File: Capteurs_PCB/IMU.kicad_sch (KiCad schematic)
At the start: 3 parts, among them U3 LSM6DSL

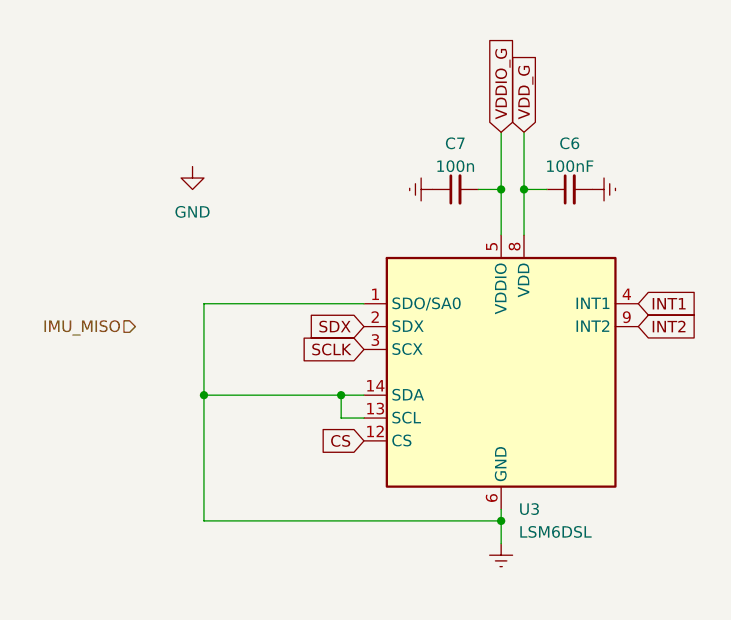
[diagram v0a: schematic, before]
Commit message: Modif PCB
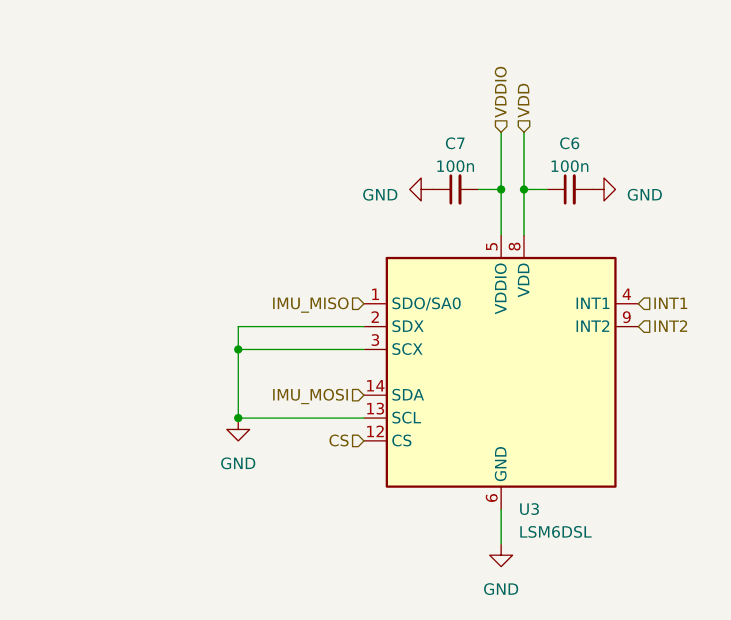
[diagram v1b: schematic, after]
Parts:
- C6: value 100nF -> 100n
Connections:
- net SCLK is gone; now on net GND: U3.3 (SCX)
- net SDX is gone; now on net GND: U3.2 (SDX)
- net GND: now also C6.2, C7.1, U3.13 (SCL), U3.6 (GND), U3.7 (GND)
- net IMU_MISO: now also U3.1 (SDO/SA0)
- removed net Earth: C6.2, C7.1, U3.1 (SDO/SA0), U3.13 (SCL), U3.14 (SDA), U3.6 (GND), U3.7 (GND)
- net VDDIO_G renamed VDDIO
- net VDD_G renamed VDD
- new net IMU_MOSI: U3.14 (SDA)
